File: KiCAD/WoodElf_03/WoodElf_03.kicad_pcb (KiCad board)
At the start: 2 copper layers, 21.6 x 21.6 mm, 14 parts, among them T1 BlankThrough-Hole, T10 BlankThrough-Hole, T2 BlankThrough-Hole, T3 BlankThrough-Hole, T5 BlankThrough-Hole, T6 BlankThrough-Hole, T9 BlankThrough-Hole

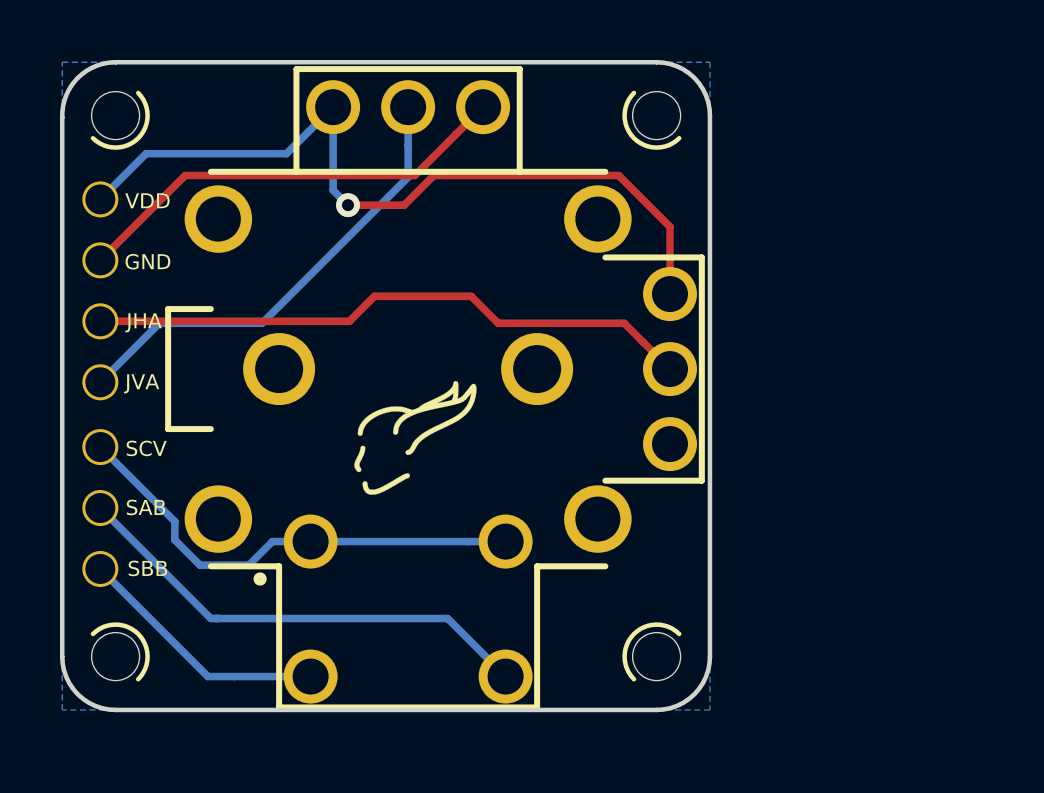
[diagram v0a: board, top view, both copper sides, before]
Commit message: working out how to mount the joystick to the sandwich
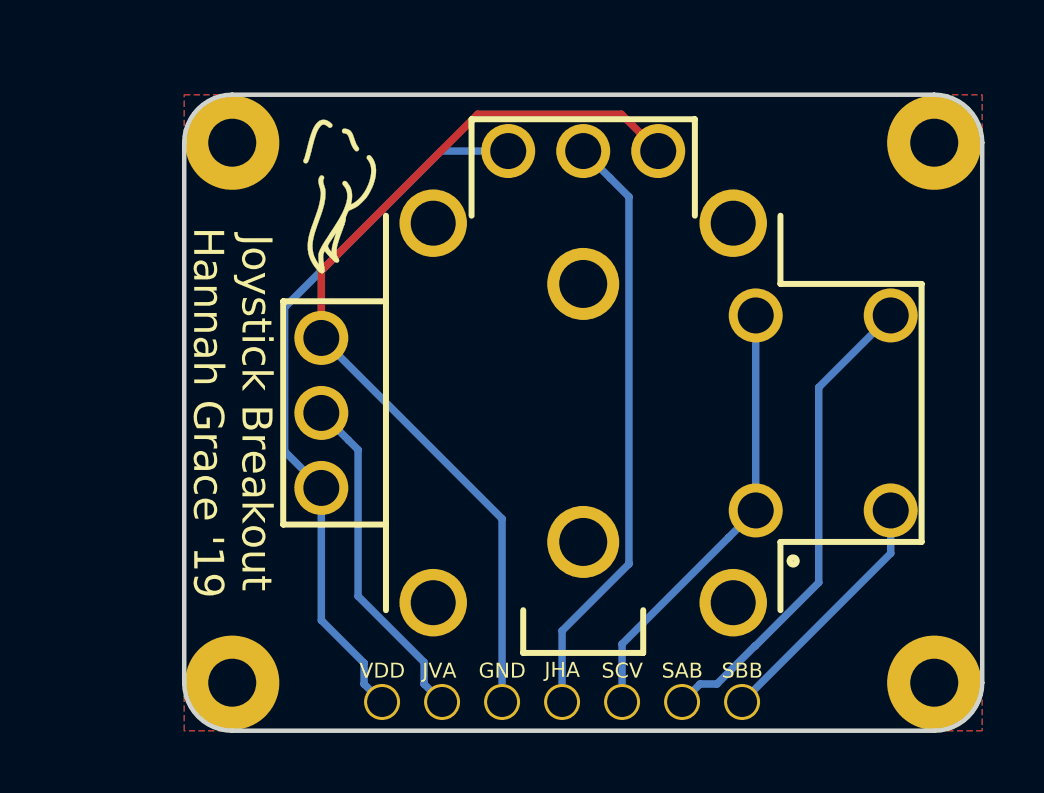
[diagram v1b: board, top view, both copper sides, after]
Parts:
- removed the Mount at (57.9, 31.5)
- removed the Mount at (57.9, 49.5)
- removed the Mount at (75.9, 49.5)
- added Mount: Mount, WoodElf_Lib:Mount, F.Cu at (61.8, 50.4)
- added Mount: Mount, WoodElf_Lib:Mount, F.Cu at (85.2, 50.4)
- added Mount: Mount, WoodElf_Lib:Mount, F.Cu at (85.2, 32.4)
- moved T1 21.8 mm to (78.8, 51.0), turned to 180 degrees
- moved T2 20.4 mm to (76.8, 51.0), turned to 180 degrees
- moved T6 19.9 mm to (72.8, 51.0), turned to 180 degrees
- moved T5 19.9 mm to (70.8, 51.0), turned to 180 degrees
- moved T3 19.4 mm to (74.8, 51.0), turned to 180 degrees
- moved T9 19.2 mm to (66.8, 51.0), turned to 180 degrees
- moved T10 15.6 mm to (68.8, 51.0), turned to 180 degrees
- moved Mount 14.2 mm to (61.8, 32.4), turned to 135 degrees
- moved G*** 9.12 mm to (64.8, 33.9), turned to 225 degrees
- moved S1 6.02 mm to (73.5, 41.4), turned to 90 degrees
- moved G*** 3.06 mm to (64.7, 34.3), turned to 135 degrees
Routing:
- net /1_1: track 14.9 -> 30.8 mm
- net /2_2: track 15.4 -> 11.3 mm
- net /3_1: track 26.6 -> 24.1 mm, vias 1 -> 0
- net /A: track 15.8 -> 14.7 mm
- added copper zone on F.Cu, net /3_1
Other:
- board size 21.6 x 21.6 mm -> 26.6 x 21.2 mm
